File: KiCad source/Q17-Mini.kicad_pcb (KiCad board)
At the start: 2 copper layers, 95 x 75 mm, 85 parts, among them J1 Input, J2-1 SPK+, J2-2 SPK-, J3-1 V+, J3-2 GND, J3-3 V-, Q1 IRF610, Q10 KSA992, Q11 BS250P, Q12 BD139, Q13 IRF610, Q14 IRF9610, Q15 FQA46N15, Q16 FQA36P15, Q2 KSA992, Q3 KSC1845, Q4 IRF9610, Q5 FQP3P20, Q6 FQP3N30, Q7 KSC1845, Q8 ZVN4206AV, Q9 BS250P, U1 OPA1641, U1' OPA1641

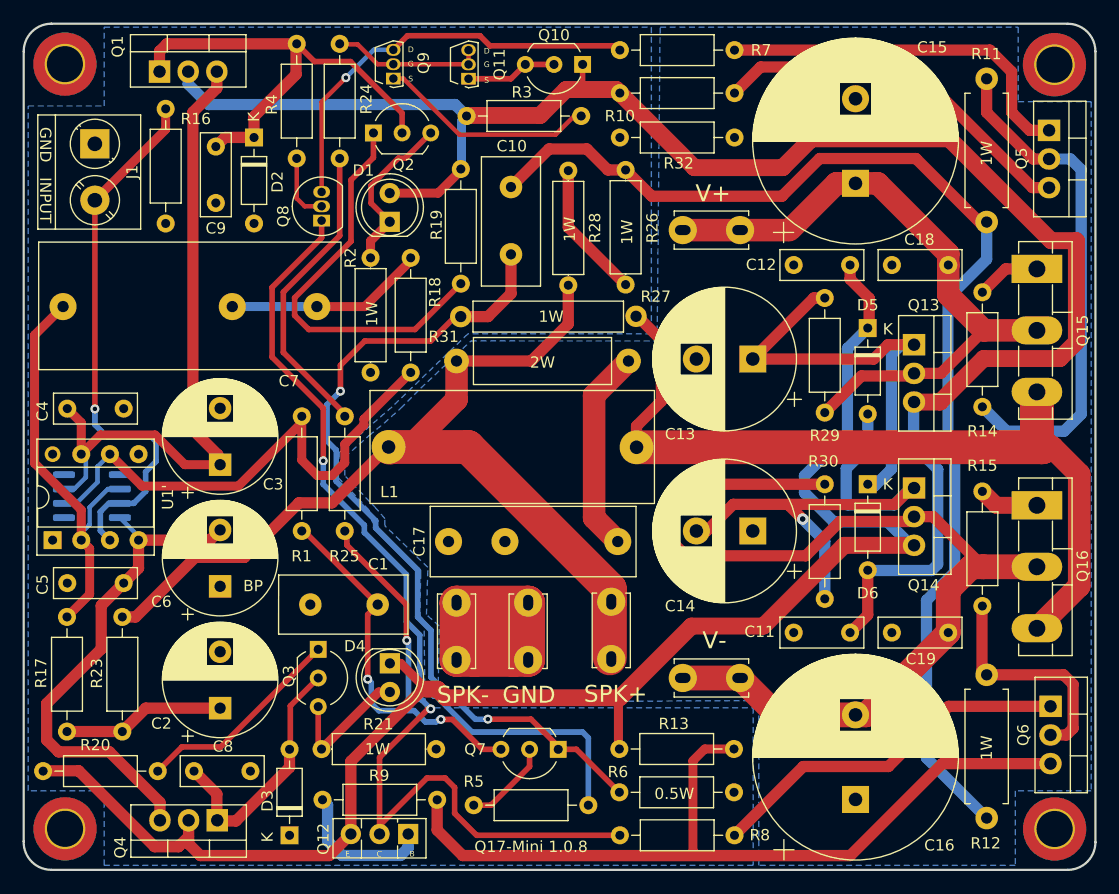
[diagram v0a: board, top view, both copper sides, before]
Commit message: PCB V1.0.8
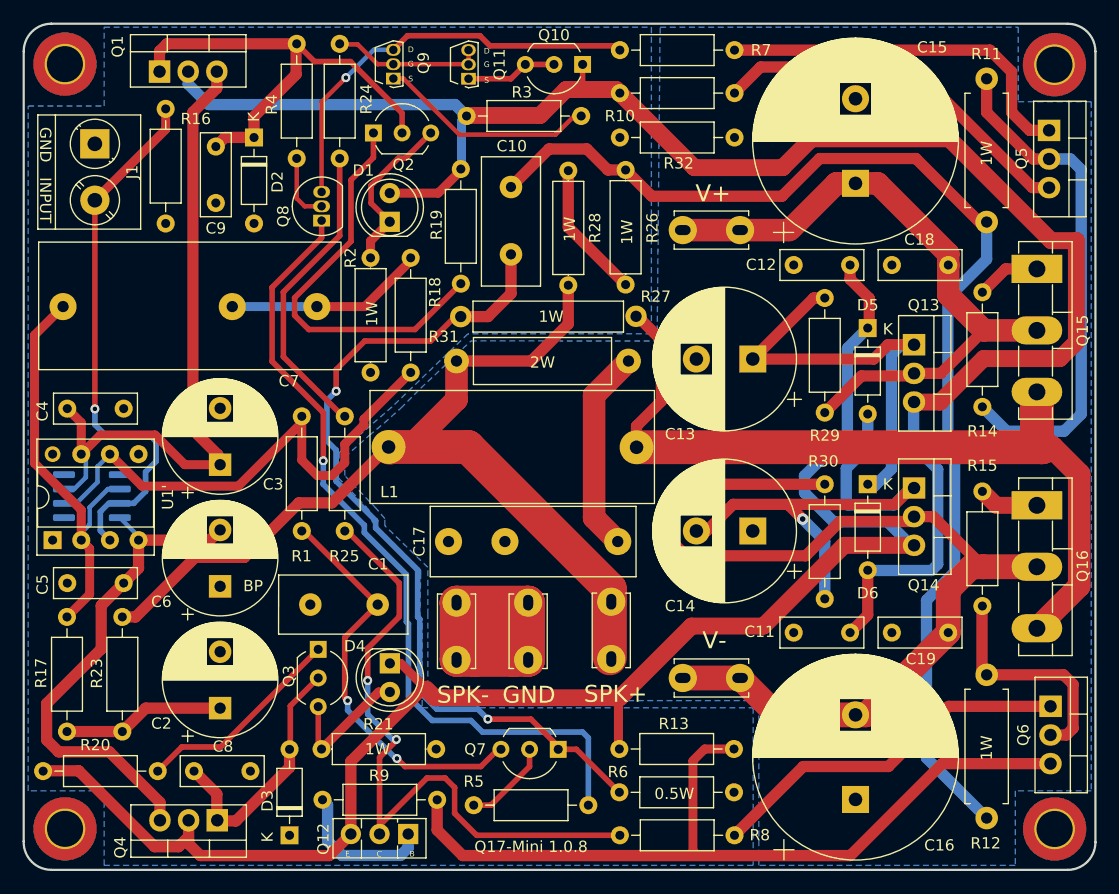
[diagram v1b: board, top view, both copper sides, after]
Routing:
- net Net-(C1-Pad1): track 31.6 -> 35.9 mm
- net Net-(C10-Pad2): track 73.8 -> 75.2 mm
- net Net-(Q8-Pad1): track 71.4 -> 72.4 mm
- net Net-(Q12-Pad2): track 59.1 -> 58.3 mm
